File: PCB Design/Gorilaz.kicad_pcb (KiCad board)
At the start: 2 copper layers, 100 x 86 mm, 57 parts, among them J1 Conn_01x13, J2 Conn_01x13, J3 Conn_01x13, J4 Conn_01x13, J5 HRO_TYPE-C-31-M-14, J6 Battery, J7 Conn_01x13, J8 Conn_01x13, J9 TC2030_SWD, M1 MountingHole_6.4mm_M6, M3 MountingHole_4.3mm_M4, M4 MountingHole_4.3mm_M4, Q2 2N7002, SW1 PWR, SW4 RST, U1 SRV05-4, U10 MAX17048, U3 BQ24075, U4 DW01A, U5 FS8205, U8 nRF52840_moko_mk08

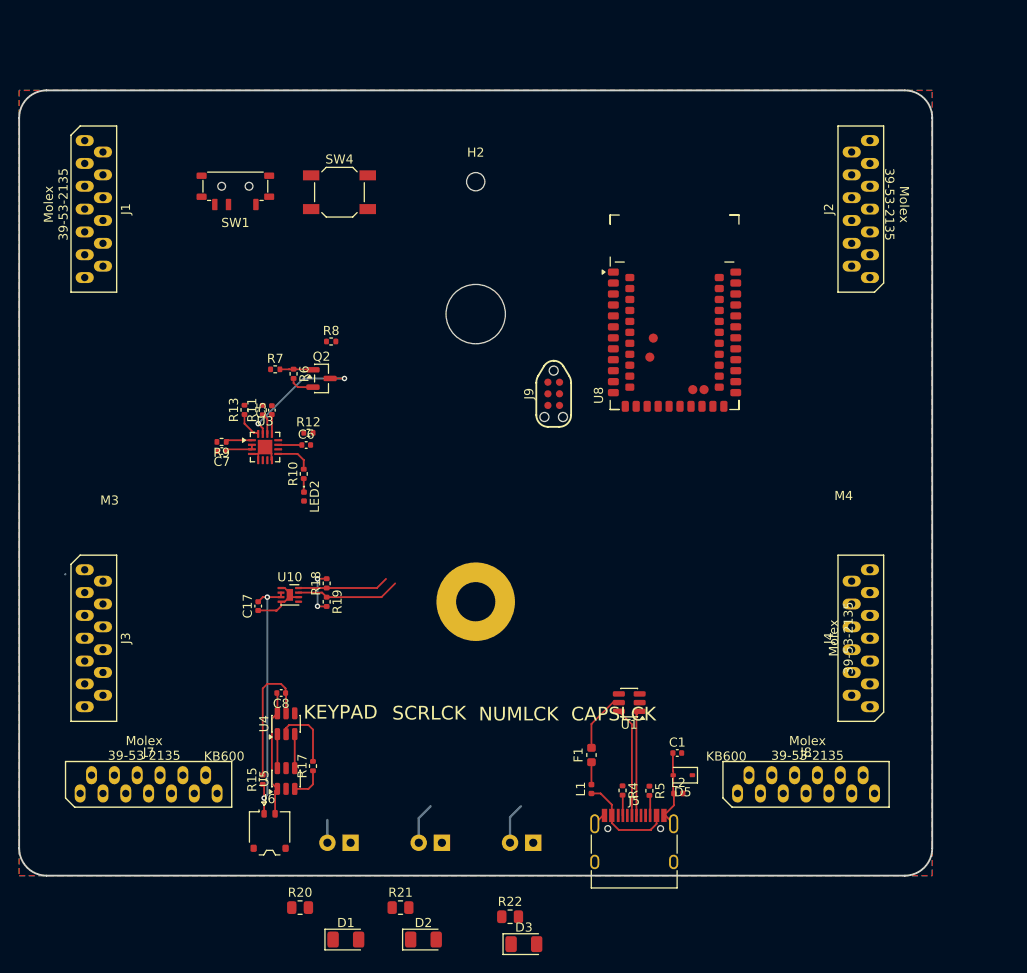
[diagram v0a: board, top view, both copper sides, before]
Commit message: v0
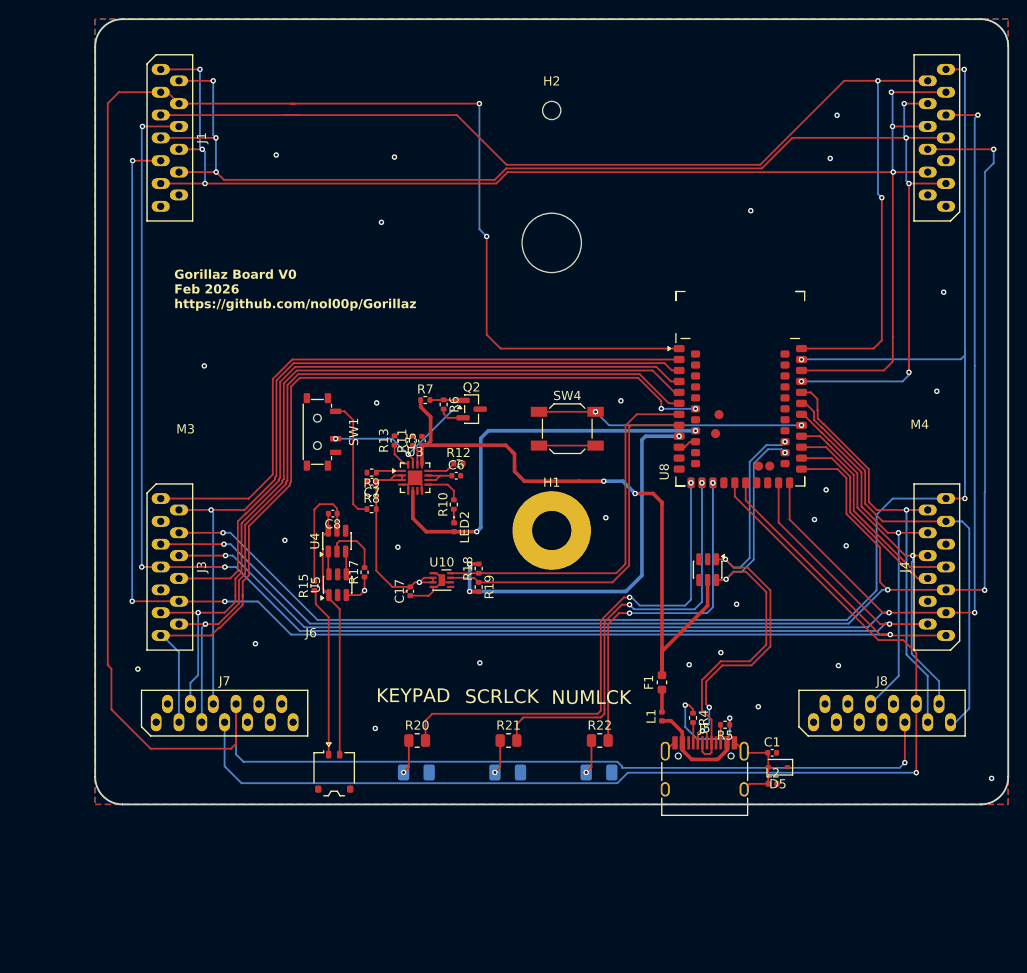
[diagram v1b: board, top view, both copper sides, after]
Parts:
- removed the D2 at (154.1, 129.4)
- removed the D3 at (144.1, 129.4)
- removed D4: LED_ALT, LED_THT:LED_D3.0mm
- removed J9: TC2030_SWD, Local:CON_TC2030_outlined
- D1, D2, D3: moved to B.Cu
- H1: moved to F.Cu
- moved SW4 36.0 mm to (157.8, 84.0)
- moved SW1 28.4 mm to (130.5, 84.4), turned to 90 degrees
- moved R20 22.3 mm to (141.4, 118.2)
- moved R15 22.0 mm to (130.2, 101.3)
- moved R17 22.0 mm to (135.7, 99.8)
- moved U5 22.0 mm to (132.7, 101.1)
- moved R21 21.8 mm to (151.4, 118.2)
- moved R22 21.7 mm to (161.4, 118.2)
- moved U4 20.8 mm to (132.6, 96.4)
- moved D3 20.5 mm to (161.3, 121.7), turned to 180 degrees
- moved D2 20.5 mm to (151.3, 121.7), turned to 180 degrees
- moved C8 20.4 mm to (132.2, 93.3)
- moved D1 19.9 mm to (141.3, 121.7), turned to 180 degrees
- moved R8 18.9 mm to (136.4, 92.9)
- moved U1 16.9 mm to (173.2, 99.5), turned to -90 degrees
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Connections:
- U8 pad 1: LED_CAPS_LOCK -> col5
- U8 pad 13: unconnected-(U8-P0.04-A-Pad13) -> LED_CAPS_LOCK
- U8 pad 14: unconnected-(U8-P0.06-Pad14) -> LED_NUM_LOCK
- U8 pad 15: unconnected-(U8-P0.11-Pad15) -> LED_SCROLL_LOCK
- U8 pad 16: unconnected-(U8-P0.08-Pad16) -> LED_KEYPAD
- U8 pad 17: unconnected-(U8-P0.09-LF-NFC-Pad17) -> col6
- U8 pad 18: unconnected-(U8-P0.10-LF-NFC-Pad18) -> col4
- U8 pad 2: LED_NUM_LOCK -> row10
- U8 pad 21: col0 -> col3
- U8 pad 22: col1 -> col2
- U8 pad 23: col2 -> col1
- U8 pad 24: col3 -> row0
- U8 pad 25: col4 -> row1
- U8 pad 26: col5 -> row2
- U8 pad 28: col6 -> row3
- U8 pad 29: unconnected-(U8-P0.20-Pad29) -> row4
- U8 pad 3: LED_SCROLL_LOCK -> row9
- U8 pad 30: unconnected-(U8-P0.21-Pad30) -> row5
- U8 pad 31: unconnected-(U8-P0.22-Pad31) -> row14
- U8 pad 32: unconnected-(U8-P0.23-Pad32) -> row13
- U8 pad 33: unconnected-(U8-P0.24-Pad33) -> col0
- U8 pad 34: unconnected-(U8-P0.25-Pad34) -> row12
- U8 pad 35: row0 -> unconnected-(U8-P1.10-LF-Pad35)
- U8 pad 36: row1 -> unconnected-(U8-P1.11-LF-Pad36)
- U8 pad 37: row2 -> unconnected-(U8-P1.12-LF-Pad37)
- U8 pad 38: row3 -> unconnected-(U8-P1.13-LF-Pad38)
- U8 pad 4: LED_KEYPAD -> row11
- U8 pad 40: row4 -> row6
- U8 pad 41: row5 -> unconnected-(U8-P1.15-LF-Pad41)
- U8 pad 44: row6 -> unconnected-(U8-P1.08-Pad44)
- U8 pad 45: row7 -> unconnected-(U8-P1.09-Pad45)
- U8 pad 5: unconnected-(U8-P0.30-LF-A-Pad5) -> row7
- U8 pad 50: row8 -> unconnected-(U8-P1.01-LF-Pad50)
- U8 pad 51: row9 -> unconnected-(U8-P1.02-LF-Pad51)
- U8 pad 52: row10 -> unconnected-(U8-P1.03-LF-Pad52)
- U8 pad 53: row11 -> unconnected-(U8-P1.04-LF-Pad53)
- U8 pad 54: row12 -> unconnected-(U8-P1.05-LF-Pad54)
- U8 pad 55: row13 -> unconnected-(U8-P1.06-LF-Pad55)
- U8 pad 56: row14 -> unconnected-(U8-P1.07-LF-Pad56)
- U8 pad 6: unconnected-(U8-P0.31-LF-A-Pad6) -> row8
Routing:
- net col5: track 0.00 -> 261.1 mm, vias 0 -> 3
- net col1: track 0.00 -> 171.3 mm, vias 0 -> 4
- net col2: track 0.00 -> 168.4 mm, vias 0 -> 4
- net col0: track 0.00 -> 168.3 mm, vias 0 -> 4
- net col4: track 0.00 -> 166.0 mm, vias 0 -> 4
- net col3: track 0.00 -> 162.8 mm, vias 0 -> 4
- net row14: track 0.00 -> 156.7 mm, vias 0 -> 8
- net row13: track 0.00 -> 153.9 mm, vias 0 -> 6
- net row12: track 0.00 -> 129.1 mm, vias 0 -> 2
- net col6: track 0.00 -> 123.5 mm, vias 0 -> 1
- net row6: track 0.00 -> 93.8 mm, vias 0 -> 2
- net row7: track 0.00 -> 90.0 mm, vias 0 -> 1
- net row9: track 0.00 -> 89.4 mm, vias 0 -> 1
- net row8: track 0.00 -> 89.3 mm, vias 0 -> 1
- net row11: track 0.00 -> 74.5 mm
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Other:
- board text added: "Gorillaz Board V0 Feb 2026 https://github.com/nol00p/Gorillaz"
- board text removed: "CAPSLCK"
- board text removed: "KB600"
- board text removed: "Molex 39-53-2135"
- board text removed: "Top Left of Board X: 100 Y: 50"
